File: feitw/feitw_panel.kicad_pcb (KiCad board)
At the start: 2 copper layers, 20.3 x 128.5 mm, 0 parts

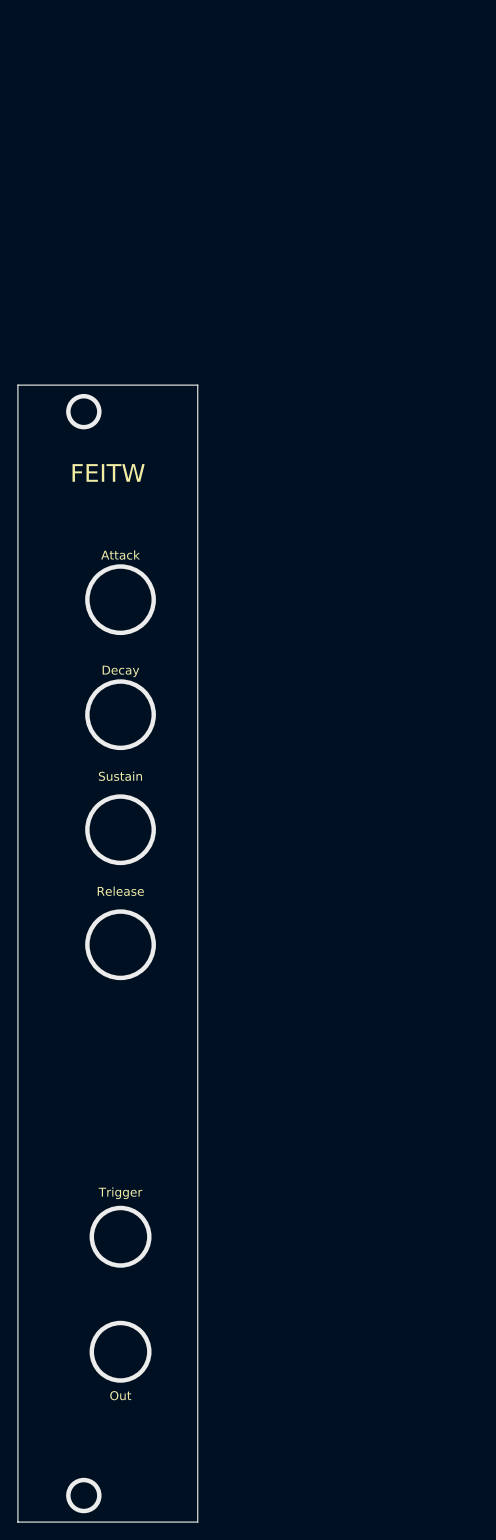
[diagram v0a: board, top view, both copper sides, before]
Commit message: feitw bugfixes
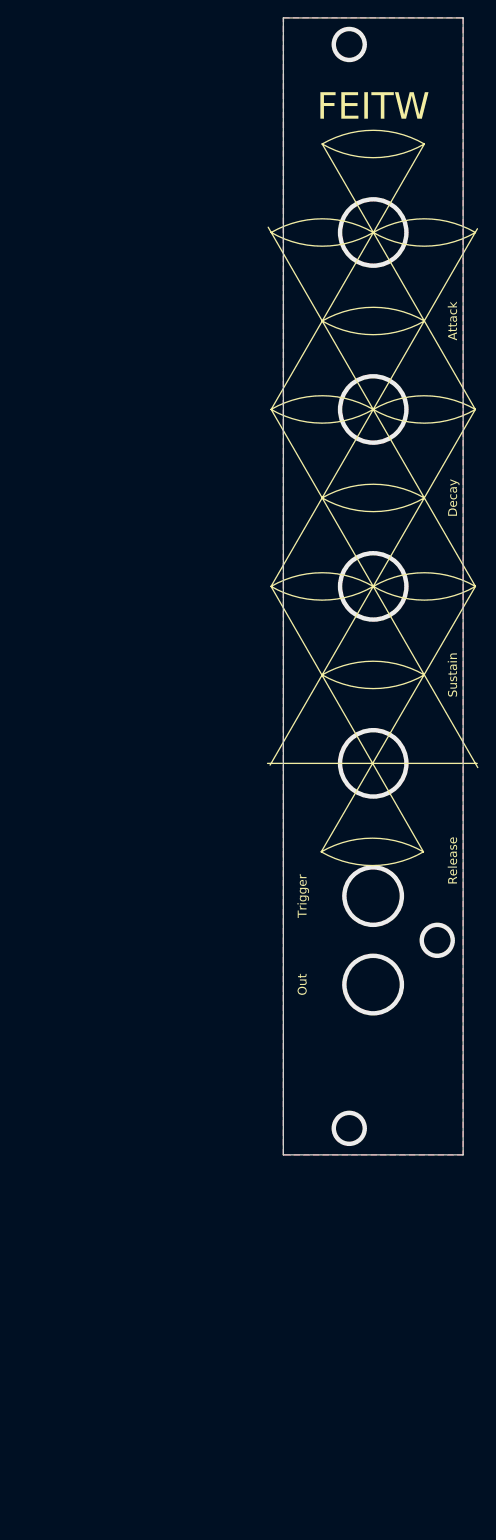
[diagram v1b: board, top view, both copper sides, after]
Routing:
- net GND: vias 6 -> 9
- net (no net): vias 2 -> 0
- added copper zone on B.Cu, net GND
- added copper zone on F.Cu, net GND
